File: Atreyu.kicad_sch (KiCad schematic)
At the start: 124 parts, among them SW1 SW_Push, U1 Elite-C

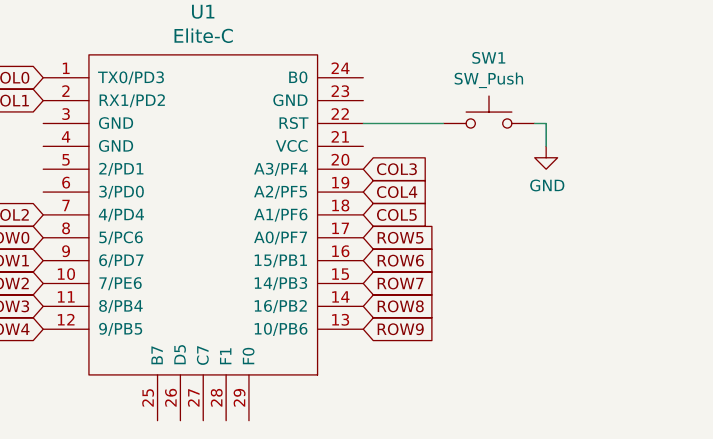
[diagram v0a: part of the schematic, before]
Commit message: Completed v0.1.
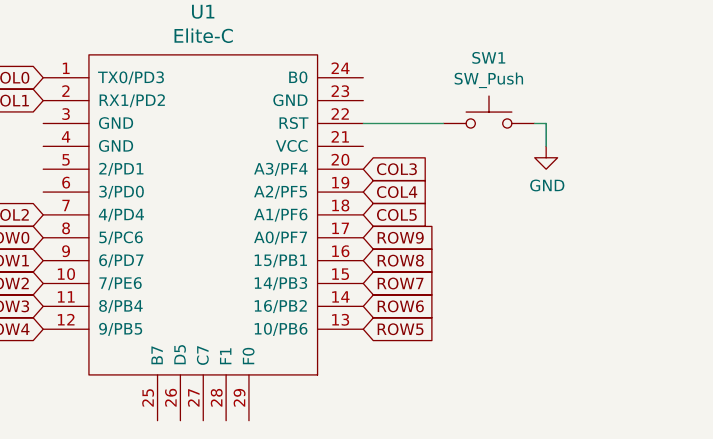
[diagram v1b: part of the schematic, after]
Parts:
- D1, D10, D11, D12, D13, D14, D15, D16, D17, D18, D19, D2, D20, D21, D22, D23, D24, D25, D26, D27, D28, D29, D3, D30, D31, D32, D33, D34, D35, D36, D37, D38, D39, D4, D40, D41, D42, D43, D44, D45, D46, D47, D48, D49, D5, D50, D51, D52, D53, D54, D55, D56, D57, D58, D59, D6, D60, D7, D8, D9: footprint Keebio-Parts:D3_hybrid_common_hole -> Atreyu:D3_hybrid_common_hole
- SW1: footprint random-keyboard-parts:SKQG-1155865 -> kbd:ResetSW_1side
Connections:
- net ROW5: now also U1.13 (10/PB6); no longer U1.17 (A0/PF7)
- net ROW6: now also U1.14 (16/PB2); no longer U1.16 (15/PB1)
- net ROW8: now also U1.16 (15/PB1); no longer U1.14 (16/PB2)
- net ROW9: now also U1.17 (A0/PF7); no longer U1.13 (10/PB6)
